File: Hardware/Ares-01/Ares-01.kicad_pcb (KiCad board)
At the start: 2 copper layers, 28 parts, among them J1 BTS7960, J12 XT60, J13 TCRT5000_1, J14 TCRT5000_2, J15 TCRT5000_3, J2 BTS7960, J3 Sharp, J4 Sharp, J5 Sharp, J6 Sharp, J7 Sharp, J8 Qtr8a, J9 Ssd1306 Arduino Pic, SW1 Switch, SW2 SW_Push, SW3 SW_Push, U1 L7805, U2 AMS1117, U3 CD74HC4067M

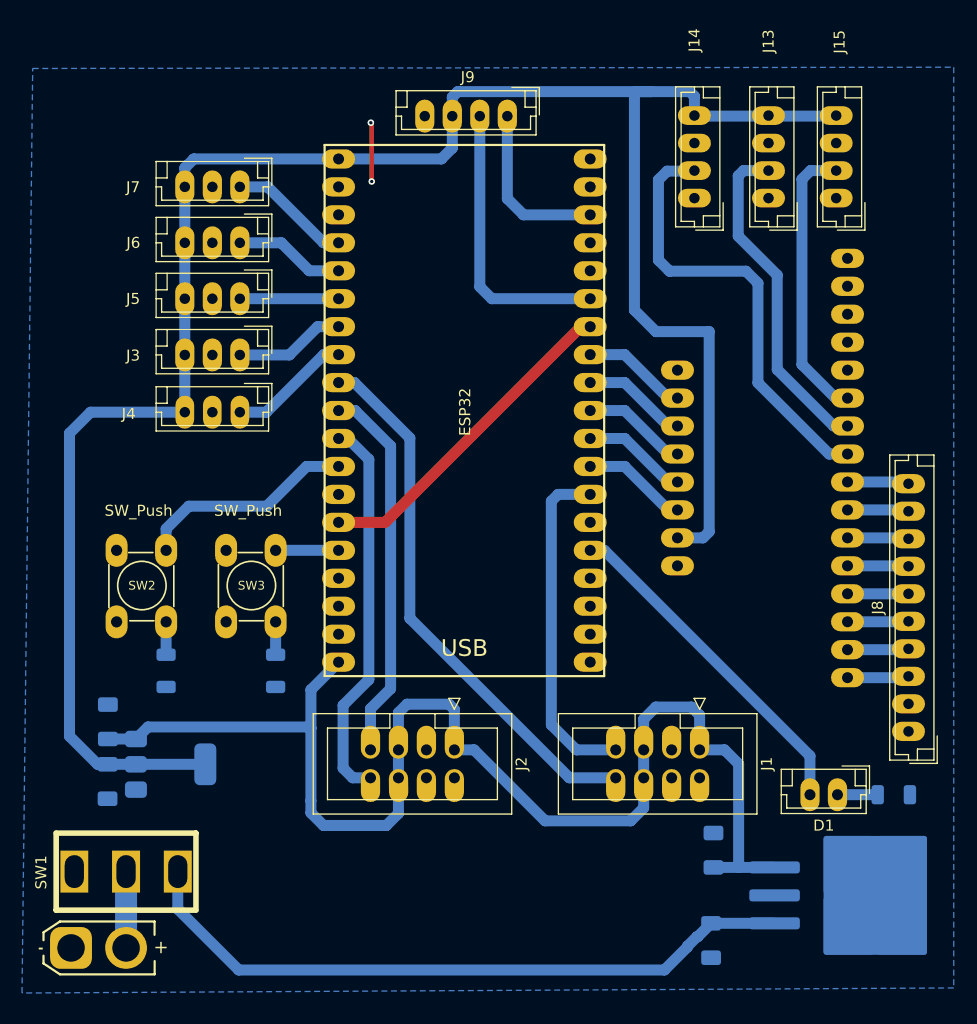
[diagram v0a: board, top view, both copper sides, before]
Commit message: version 3 del pcb
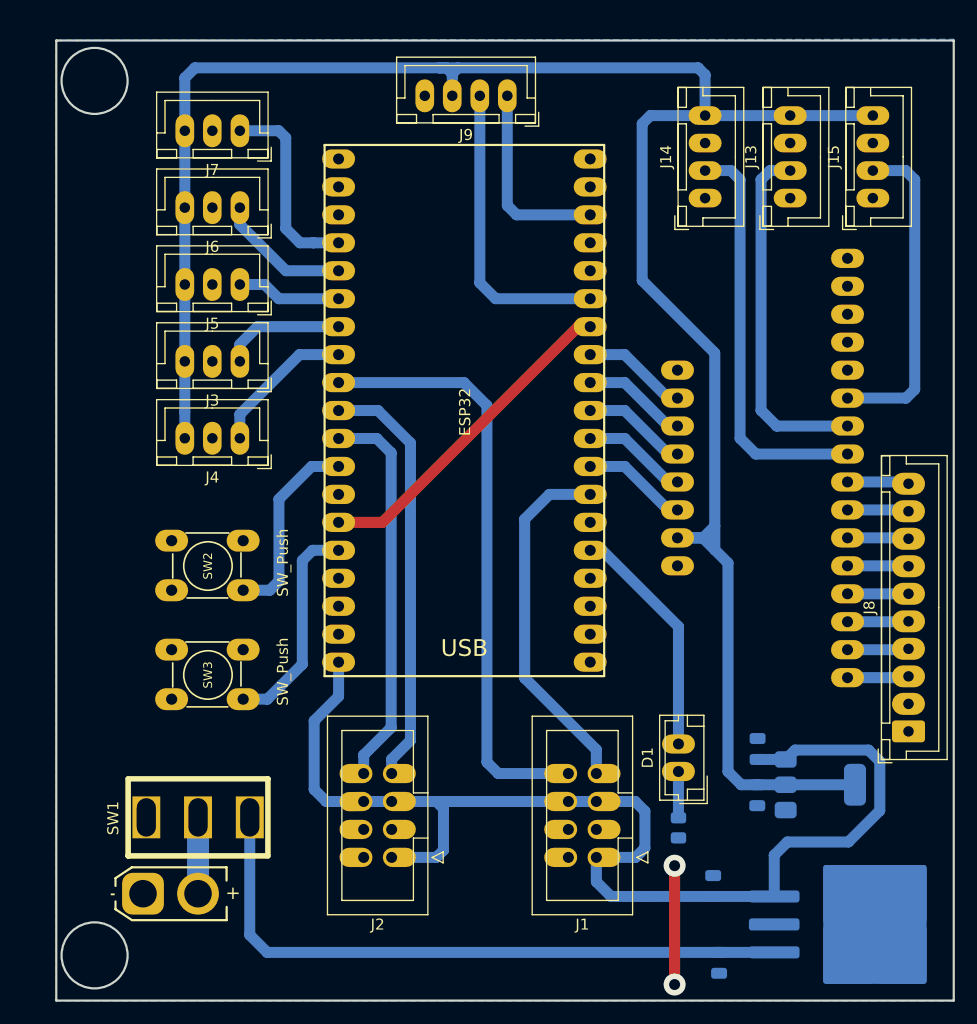
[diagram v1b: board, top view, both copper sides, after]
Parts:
- removed R12, R13: 220, Resistor_SMD:R_1206_3216Metric
- C2, C3, C4, C5: footprint Capacitor_SMD:C_1206_3216Metric_Pad1.33x1.80mm_HandSolder -> Capacitor_SMD:C_0805_2012Metric
- J12: value XT60 -> XT30
- J13, J14, J15, J9: footprint Connector_JST:JST_EH_B4B-EH-A_1x04_P2.50mm_Vertical -> Connector_JST:JST_XH_B4B-XH-A_1x04_P2.50mm_Vertical
- J3, J4, J5, J6, J7: footprint Connector_JST:JST_EH_B3B-EH-A_1x03_P2.50mm_Vertical -> Connector_JST:JST_XH_B3B-XH-A_1x03_P2.50mm_Vertical
- J8: footprint Connector_JST:JST_EH_B10B-EH-A_1x10_P2.50mm_Vertical -> Connector_JST:JST_XH_B10B-XH-A_1x10_P2.50mm_Vertical
- R11: footprint Resistor_SMD:R_1206_3216Metric -> Resistor_SMD:R_0805_2012Metric
- moved C4 59.1 mm to (209.2, 93.0)
- moved U2 59.1 mm to (214.9, 96.2)
- moved C5 59.0 mm to (209.2, 97.2)
- moved R11 19.8 mm to (202.1, 100.2), turned to 90 degrees
- moved D1 14.6 mm to (202.1, 95.0), turned to 90 degrees
- moved J1 13.5 mm to (194.6, 102.8), turned to 180 degrees
- moved SW2 11.5 mm to (162.5, 74.1), turned to -90 degrees
- moved J2 11.3 mm to (176.0, 102.8), turned to 180 degrees
- moved SW3 9.16 mm to (162.5, 84.0), turned to -90 degrees
- moved J12 8.19 mm to (153.4, 106.2)
- moved SW1 8.19 mm to (158.4, 99.2)
- moved J7 5.10 mm to (162.2, 36.8)
- moved J15 3.33 mm to (219.7, 43.0)
- moved C2 3.25 mm to (205.2, 105.5)
- moved J6 3.20 mm to (162.2, 43.8)
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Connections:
- ESP32 pad 1: 3.3V -> unconnected-(ESP32-3v3-Pad1)
- SW2 pad 2: Net-(R12-Pad2) -> GND
- SW3 pad 2: Net-(R13-Pad2) -> GND
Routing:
- net B2: track 5.72 -> 19.8 mm
- net LED: track 31.2 -> 21.6 mm
- net OUT5: track 11.1 -> 18.1 mm
- net GND: track 35.6 -> 41.0 mm
- net LPWM_2: track 49.7 -> 54.6 mm
- net RPWM_1: track 34.4 -> 38.5 mm
- net OUT_C: track 25.7 -> 29.6 mm
- net OUT_B: track 40.7 -> 37.4 mm
- net Net-(R13-Pad2): track 2.99 -> 0.00 mm
- net Net-(R12-Pad2): track 2.99 -> 0.00 mm
- net Net-(SW1-A): track 61.7 -> 59.0 mm
- net B1: track 20.0 -> 17.7 mm
- net OUT2: track 11.1 -> 13.4 mm
- net OUT4: track 10.0 -> 12.3 mm
- net SDA: track 15.6 -> 17.9 mm
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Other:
- board outline added: 81.5 x 87.2 mm
